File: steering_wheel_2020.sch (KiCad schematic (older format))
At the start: 38 parts, among them J1 VEHICLE, J10 Conn_01x15, J11 Conn_01x15, J12 ALT_PWR, J2 DEBUG, J3 Conn_01x15, J4 Conn_01x13, J5 Conn_01x15, J6 Conn_01x13, J7 Conn_01x15, J8 Conn_01x13, J9 Conn_01x15, U1 STM32F103R8Tx, U2 SN65HVD232, U3 LD1117S33CTR, Y1 8MHz

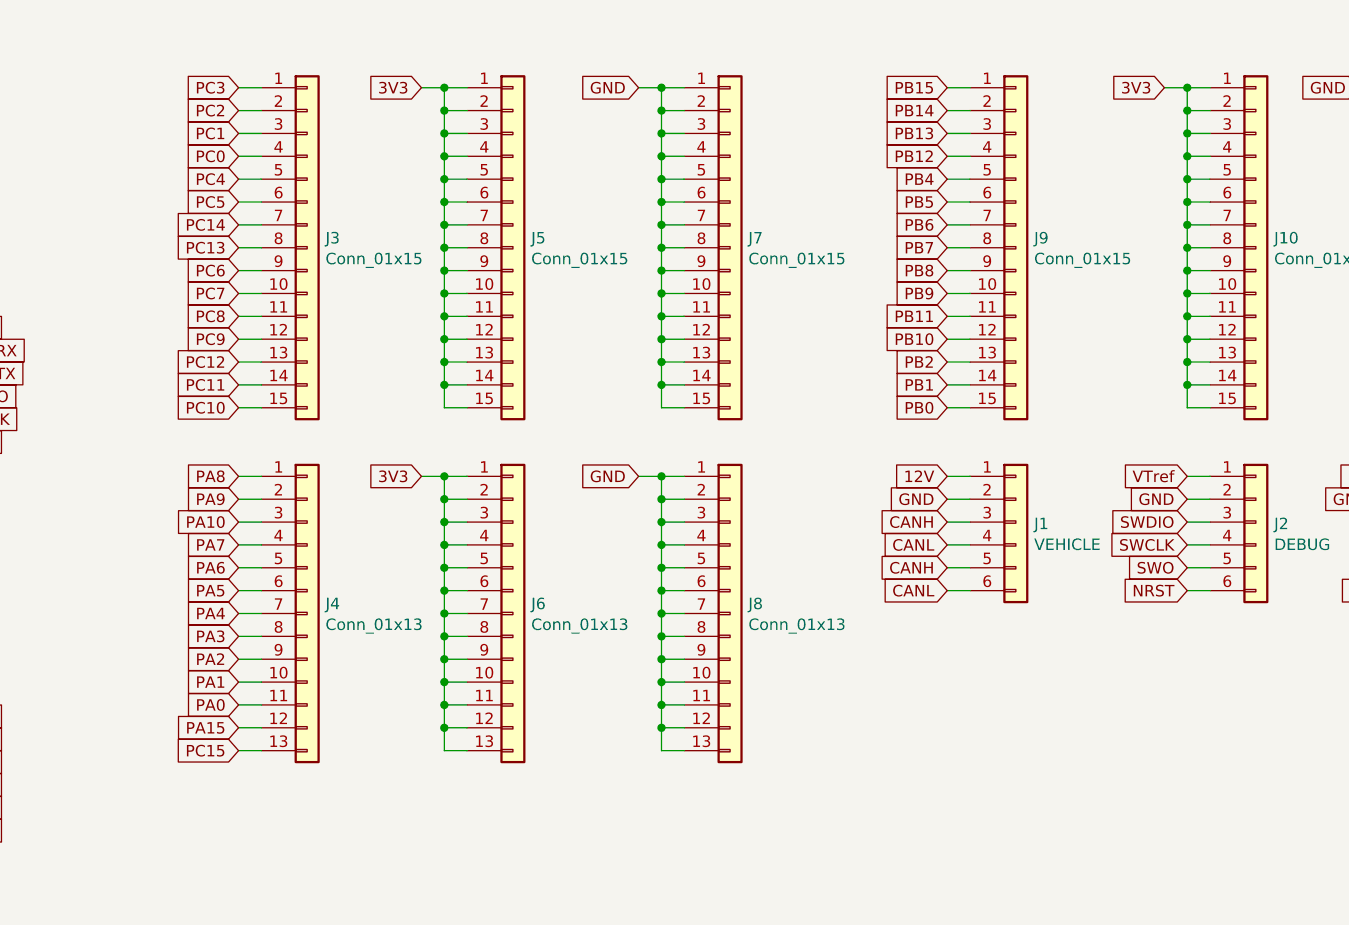
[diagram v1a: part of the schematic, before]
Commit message: routing mostly done
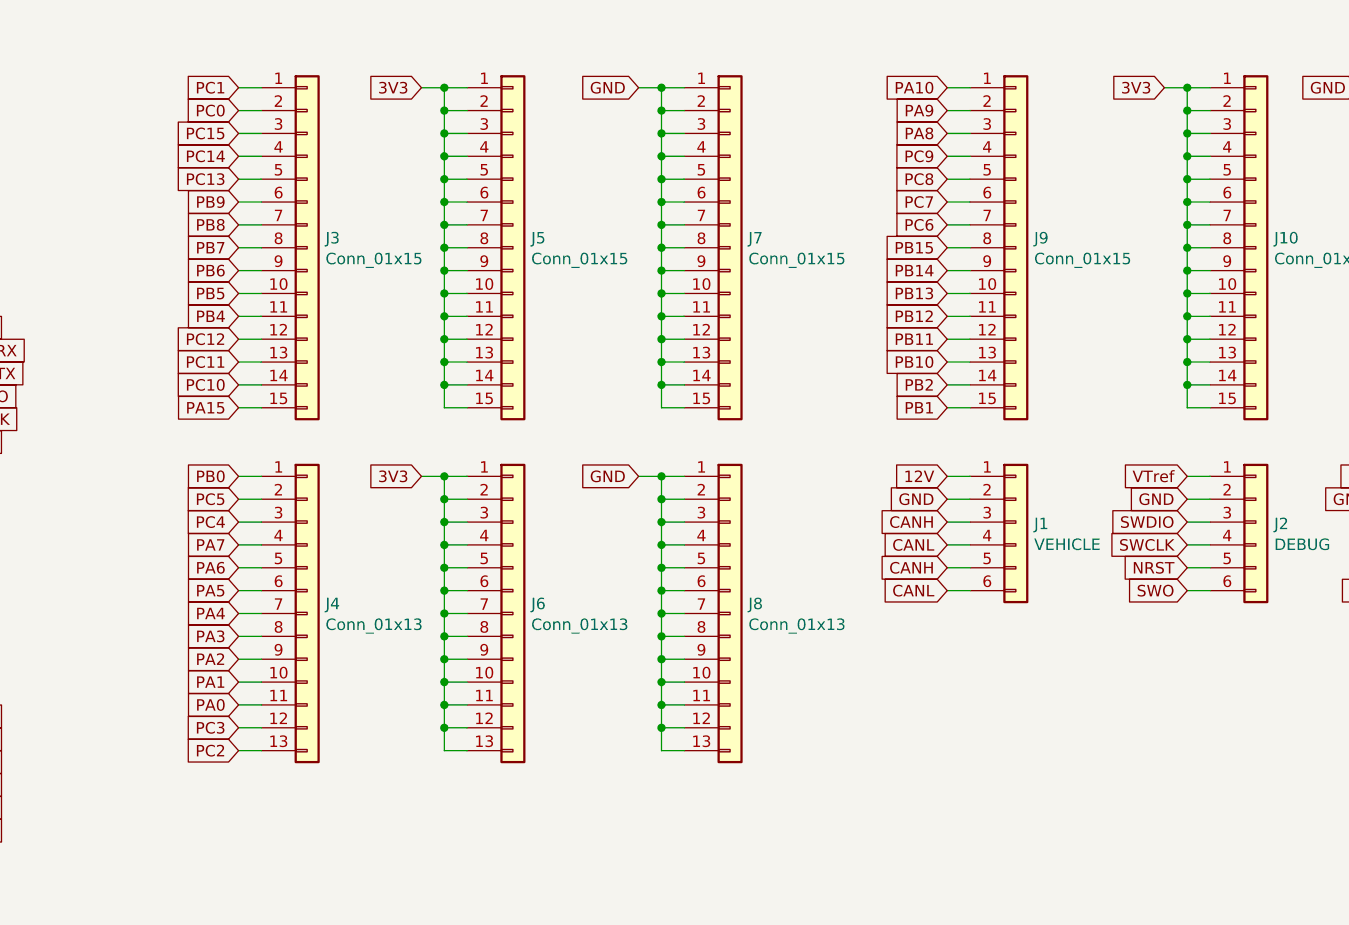
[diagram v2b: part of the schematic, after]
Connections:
- net NRST: now also J2.5 (Pin_5); no longer J2.6 (Pin_6)
- net PA10: now also J9.1 (Pin_1); no longer J4.3 (Pin_3)
- net PA15: now also J3.15 (Pin_15); no longer J4.12 (Pin_12)
- net PA8: now also J9.3 (Pin_3); no longer J4.1 (Pin_1)
- net PA9: now also J9.2 (Pin_2); no longer J4.2 (Pin_2)
- net PB0: now also J4.1 (Pin_1); no longer J9.15 (Pin_15)
- net PB1: now also J9.15 (Pin_15); no longer J9.14 (Pin_14)
- net PB10: now also J9.13 (Pin_13); no longer J9.12 (Pin_12)
- net PB11: now also J9.12 (Pin_12); no longer J9.11 (Pin_11)
- net PB12: now also J9.11 (Pin_11); no longer J9.4 (Pin_4)
- net PB13: now also J9.10 (Pin_10); no longer J9.3 (Pin_3)
- net PB14: now also J9.9 (Pin_9); no longer J9.2 (Pin_2)
- net PB15: now also J9.8 (Pin_8); no longer J9.1 (Pin_1)
- net PB2: now also J9.14 (Pin_14); no longer J9.13 (Pin_13)
- net PB4: now also J3.11 (Pin_11); no longer J9.5 (Pin_5)
- net PB5: now also J3.10 (Pin_10); no longer J9.6 (Pin_6)
- net PB6: now also J3.9 (Pin_9); no longer J9.7 (Pin_7)
- net PB7: now also J3.8 (Pin_8); no longer J9.8 (Pin_8)
- net PB8: now also J3.7 (Pin_7); no longer J9.9 (Pin_9)
- net PB9: now also J3.6 (Pin_6); no longer J9.10 (Pin_10)
- net PC0: now also J3.2 (Pin_2); no longer J3.4 (Pin_4)
- net PC1: now also J3.1 (Pin_1); no longer J3.3 (Pin_3)
- net PC10: now also J3.14 (Pin_14); no longer J3.15 (Pin_15)
- net PC11: now also J3.13 (Pin_13); no longer J3.14 (Pin_14)
- net PC12: now also J3.12 (Pin_12); no longer J3.13 (Pin_13)
- net PC13: now also J3.5 (Pin_5); no longer J3.8 (Pin_8)
- net PC14: now also J3.4 (Pin_4); no longer J3.7 (Pin_7)
- net PC15: now also J3.3 (Pin_3); no longer J4.13 (Pin_13)
- net PC2: now also J4.13 (Pin_13); no longer J3.2 (Pin_2)
- net PC3: now also J4.12 (Pin_12); no longer J3.1 (Pin_1)
- net PC4: now also J4.3 (Pin_3); no longer J3.5 (Pin_5)
- net PC5: now also J4.2 (Pin_2); no longer J3.6 (Pin_6)
- net PC6: now also J9.7 (Pin_7); no longer J3.9 (Pin_9)
- net PC7: now also J9.6 (Pin_6); no longer J3.10 (Pin_10)
- net PC8: now also J9.5 (Pin_5); no longer J3.11 (Pin_11)
- net PC9: now also J9.4 (Pin_4); no longer J3.12 (Pin_12)
- net SWO: now also J2.6 (Pin_6); no longer J2.5 (Pin_5)
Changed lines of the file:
@@
 Text GLabel 9200 2950 0    50   Input ~ 0
 SWCLK
+Text GLabel 9200 3150 0    50   Input ~ 0
+SWO
 Text GLabel 9200 3050 0    50   Input ~ 0
-SWO
-Text GLabel 9200 3150 0    50   Input ~ 0
 NRST
 Text GLabel 9200 2750 0    50   Input ~ 0
@@
 Wire Wire Line
 	6900 1050 6900 1150
+Text GLabel 5050 1050 0    50   Input ~ 0
+PC0
+Text GLabel 5050 950  0    50   Input ~ 0
+PC1
+Text GLabel 5050 3850 0    50   Input ~ 0
+PC2
+Text GLabel 5050 3750 0    50   Input ~ 0
+PC3
+Text GLabel 5050 2850 0    50   Input ~ 0
+PC4
+Text GLabel 5050 2750 0    50   Input ~ 0
+PC5
+Text GLabel 8150 1550 0    50   Input ~ 0
+PC6
+Text GLabel 8150 1450 0    50   Input ~ 0
+PC7
+Text GLabel 8150 1350 0    50   Input ~ 0
+PC8
+Text GLabel 8150 1250 0    50   Input ~ 0
+PC9
+Text GLabel 5050 2250 0    50   Input ~ 0
+PC10
+Text GLabel 5050 2150 0    50   Input ~ 0
+PC11
+Text GLabel 5050 2050 0    50   Input ~ 0
+PC12
+Text GLabel 5050 1350 0    50   Input ~ 0
+PC13
 Text GLabel 5050 1250 0    50   Input ~ 0
-PC0
-Text GLabel 5050 1150 0    50   Input ~ 0
-PC1
-Text GLabel 5050 1050 0    50   Input ~ 0
-PC2
-Text GLabel 5050 950  0    50   Input ~ 0
-PC3
-Text GLabel 5050 1350 0    50   Input ~ 0
-PC4
-Text GLabel 5050 1450 0    50   Input ~ 0
-PC5
-Text GLabel 5050 1750 0    50   Input ~ 0
-PC6
-Text GLabel 5050 1850 0    50   Input ~ 0
-PC7
-Text GLabel 5050 1950 0    50   Input ~ 0
-PC8
-Text GLabel 5050 2050 0    50   Input ~ 0
-PC9
-Text GLabel 5050 2350 0    50   Input ~ 0
-PC10
-Text GLabel 5050 2250 0    50   Input ~ 0
-PC11
-Text GLabel 5050 2150 0    50   Input ~ 0
-PC12
-Text GLabel 5050 1650 0    50   Input ~ 0
-PC13
-Text GLabel 5050 1550 0    50   Input ~ 0
 PC14
-Wire Wire Line
-	5050 1450 5150 1450
-Wire Wire Line
-	5150 1350 5050 1350
 $Comp
 L Connector_Generic:Conn_01x15 J9
@@
 Wire Wire Line
 	10050 1050 10050 1150
+Text GLabel 5050 2650 0    50   Input ~ 0
+PB0
 Text GLabel 8150 2350 0    50   Input ~ 0
-PB0
+PB1
 Text GLabel 8150 2250 0    50   Input ~ 0
-PB1
+PB2
+Text GLabel 5050 1950 0    50   Input ~ 0
+PB4
+Text GLabel 5050 1850 0    50   Input ~ 0
+PB5
+Text GLabel 5050 1750 0    50   Input ~ 0
+PB6
+Text GLabel 5050 1650 0    50   Input ~ 0
+PB7
+Text GLabel 5050 1550 0    50   Input ~ 0
+PB8
+Text GLabel 5050 1450 0    50   Input ~ 0
+PB9
 Text GLabel 8150 2150 0    50   Input ~ 0
-PB2
-Text GLabel 8150 1350 0    50   Input ~ 0
-PB4
-Text GLabel 8150 1450 0    50   Input ~ 0
-PB5
-Text GLabel 8150 1550 0    50   Input ~ 0
-PB6
+PB10
+Text GLabel 8150 2050 0    50   Input ~ 0
+PB11
+Text GLabel 8150 1950 0    50   Input ~ 0
+PB12
+Text GLabel 8150 1850 0    50   Input ~ 0
+PB13
+Text GLabel 8150 1750 0    50   Input ~ 0
+PB14
 Text GLabel 8150 1650 0    50   Input ~ 0
-PB7
-Text GLabel 8150 1750 0    50   Input ~ 0
-PB8
-Text GLabel 8150 1850 0    50   Input ~ 0
-PB9
-Text GLabel 8150 2050 0    50   Input ~ 0
-PB10
-Text GLabel 8150 1950 0    50   Input ~ 0
-PB11
-Text GLabel 8150 1250 0    50   Input ~ 0
-PB12
-Text GLabel 8150 1150 0    50   Input ~ 0
-PB13
-Text GLabel 8150 1050 0    50   Input ~ 0
-PB14
-Text GLabel 8150 950  0    50   Input ~ 0
 PB15
 $Comp
@@
 Text GLabel 5050 2950 0    50   Input ~ 0
 PA7
-Text GLabel 5050 2650 0    50   Input ~ 0
+Text GLabel 8150 1150 0    50   Input ~ 0
 PA8
-Text GLabel 5050 2750 0    50   Input ~ 0
+Text GLabel 8150 1050 0    50   Input ~ 0
 PA9
-Text GLabel 5050 2850 0    50   Input ~ 0
+Text GLabel 8150 950  0    50   Input ~ 0
 PA10
-Text GLabel 5050 3750 0    50   Input ~ 0
+Text GLabel 5050 2350 0    50   Input ~ 0
 PA15
-Text GLabel 5050 3850 0    50   Input ~ 0
+Text GLabel 5050 1150 0    50   Input ~ 0
 PC15
-Wire Wire Line
-	5050 3750 5150 3750
-Wire Wire Line
-	5150 3850 5050 3850
 Text GLabel 5850 2650 0    50   Input ~ 0
 3V3
@@
 Wire Wire Line
 	9200 2750 9300 2750
-Wire Wire Line
-	9200 2850 9300 2850
-Wire Wire Line
-	9200 2950 9300 2950
-Wire Wire Line
-	9200 3050 9300 3050
-Wire Wire Line
-	9200 3150 9300 3150
 $Comp
 L Connector_Generic:Conn_01x02 J12
@@
 	10100 3150 10200 3150
 Wire Wire Line
+	8150 950  8250 950
+Wire Wire Line
+	8150 1050 8250 1050
+Wire Wire Line
+	8150 1150 8250 1150
+Wire Wire Line
+	8150 1250 8250 1250
+Wire Wire Line
+	8150 1350 8250 1350
+Wire Wire Line
+	8150 1450 8250 1450
+Wire Wire Line
+	8150 1550 8250 1550
+Wire Wire Line
+	5050 1750 5150 1750
+Wire Wire Line
+	8150 1650 8250 1650
+Wire Wire Line
+	8150 1750 8250 1750
+Wire Wire Line
+	8150 1850 8250 1850
+Wire Wire Line
+	8150 1950 8250 1950
+Wire Wire Line
+	8150 2050 8250 2050
+Wire Wire Line
+	8150 2150 8250 2150
+Wire Wire Line
+	8150 2250 8250 2250
+Wire Wire Line
+	8150 2350 8250 2350
+Wire Wire Line
+	5050 2650 5150 2650
+Wire Wire Line
+	5050 2750 5150 2750
+Wire Wire Line
+	5050 2850 5150 2850
+Wire Wire Line
+	5050 2950 5150 2950
+Wire Wire Line
+	5050 3050 5150 3050
+Wire Wire Line
+	5050 3150 5150 3150
+Wire Wire Line
+	5050 3250 5150 3250
+Wire Wire Line
+	5050 3350 5150 3350
+Wire Wire Line
+	5050 3450 5150 3450
+Wire Wire Line
+	5050 3550 5150 3550
+Wire Wire Line
+	5050 3650 5150 3650
+Wire Wire Line
+	5050 3750 5150 3750
+Wire Wire Line
+	5050 3850 5150 3850
+Wire Wire Line
+	5050 950  5150 950
+Wire Wire Line
+	5050 1050 5150 1050
+Wire Wire Line
+	5050 1150 5150 1150
+Wire Wire Line
 	5050 1250 5150 1250
 Wire Wire Line
-	5150 1150 5050 1150
-Wire Wire Line
-	5050 1050 5150 1050
-Wire Wire Line
-	5150 950  5050 950
+	5050 1350 5150 1350
+Wire Wire Line
+	5050 1450 5150 1450
 Wire Wire Line
 	5050 1550 5150 1550
 Wire Wire Line
-	5150 1650 5050 1650
-Wire Wire Line
-	5050 1750 5150 1750
-Wire Wire Line
-	5150 1850 5050 1850
+	5050 1650 5150 1650
+Wire Wire Line
+	5050 1850 5150 1850
 Wire Wire Line
 	5050 1950 5150 1950
 Wire Wire Line
-	5150 2050 5050 2050
-Wire Wire Line
-	5150 2250 5050 2250
+	5050 2050 5150 2050
 Wire Wire Line
 	5050 2150 5150 2150
 Wire Wire Line
+	5050 2250 5150 2250
+Wire Wire Line
 	5050 2350 5150 2350
 Wire Wire Line
-	5050 2650 5150 2650
-Wire Wire Line
-	5050 2750 5150 2750
-Wire Wire Line
-	5050 2850 5150 2850
-Wire Wire Line
-	5050 2950 5150 2950
-Wire Wire Line
-	5050 3050 5150 3050
-Wire Wire Line
-	5050 3150 5150 3150
-Wire Wire Line
-	5050 3250 5150 3250
-Wire Wire Line
-	5050 3350 5150 3350
-Wire Wire Line
-	5050 3450 5150 3450
-Wire Wire Line
-	5050 3550 5150 3550
-Wire Wire Line
-	5050 3650 5150 3650
-Wire Wire Line
-	8150 2350 8250 2350
-Wire Wire Line
-	8150 2250 8250 2250
-Wire Wire Line
-	8150 2150 8250 2150
-Wire Wire Line
-	8150 1950 8250 1950
-Wire Wire Line
-	8150 2050 8250 2050
-Wire Wire Line
-	8150 1850 8250 1850
-Wire Wire Line
-	8150 1750 8250 1750
-Wire Wire Line
-	8150 1650 8250 1650
-Wire Wire Line
-	8150 1550 8250 1550
-Wire Wire Line
-	8150 1450 8250 1450
-Wire Wire Line
-	8150 1350 8250 1350
-Wire Wire Line
-	8150 1250 8250 1250
-Wire Wire Line
-	8150 950  8250 950
-Wire Wire Line
-	8150 1050 8250 1050
-Wire Wire Line
-	8150 1150 8250 1150
+	9200 3150 9300 3150
+Wire Wire Line
+	9200 2950 9300 2950
+Wire Wire Line
+	9200 2850 9300 2850
+Wire Wire Line
+	9200 3050 9300 3050
 $EndSCHEMATC
